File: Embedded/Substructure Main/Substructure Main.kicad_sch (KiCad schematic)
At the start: 0 parts

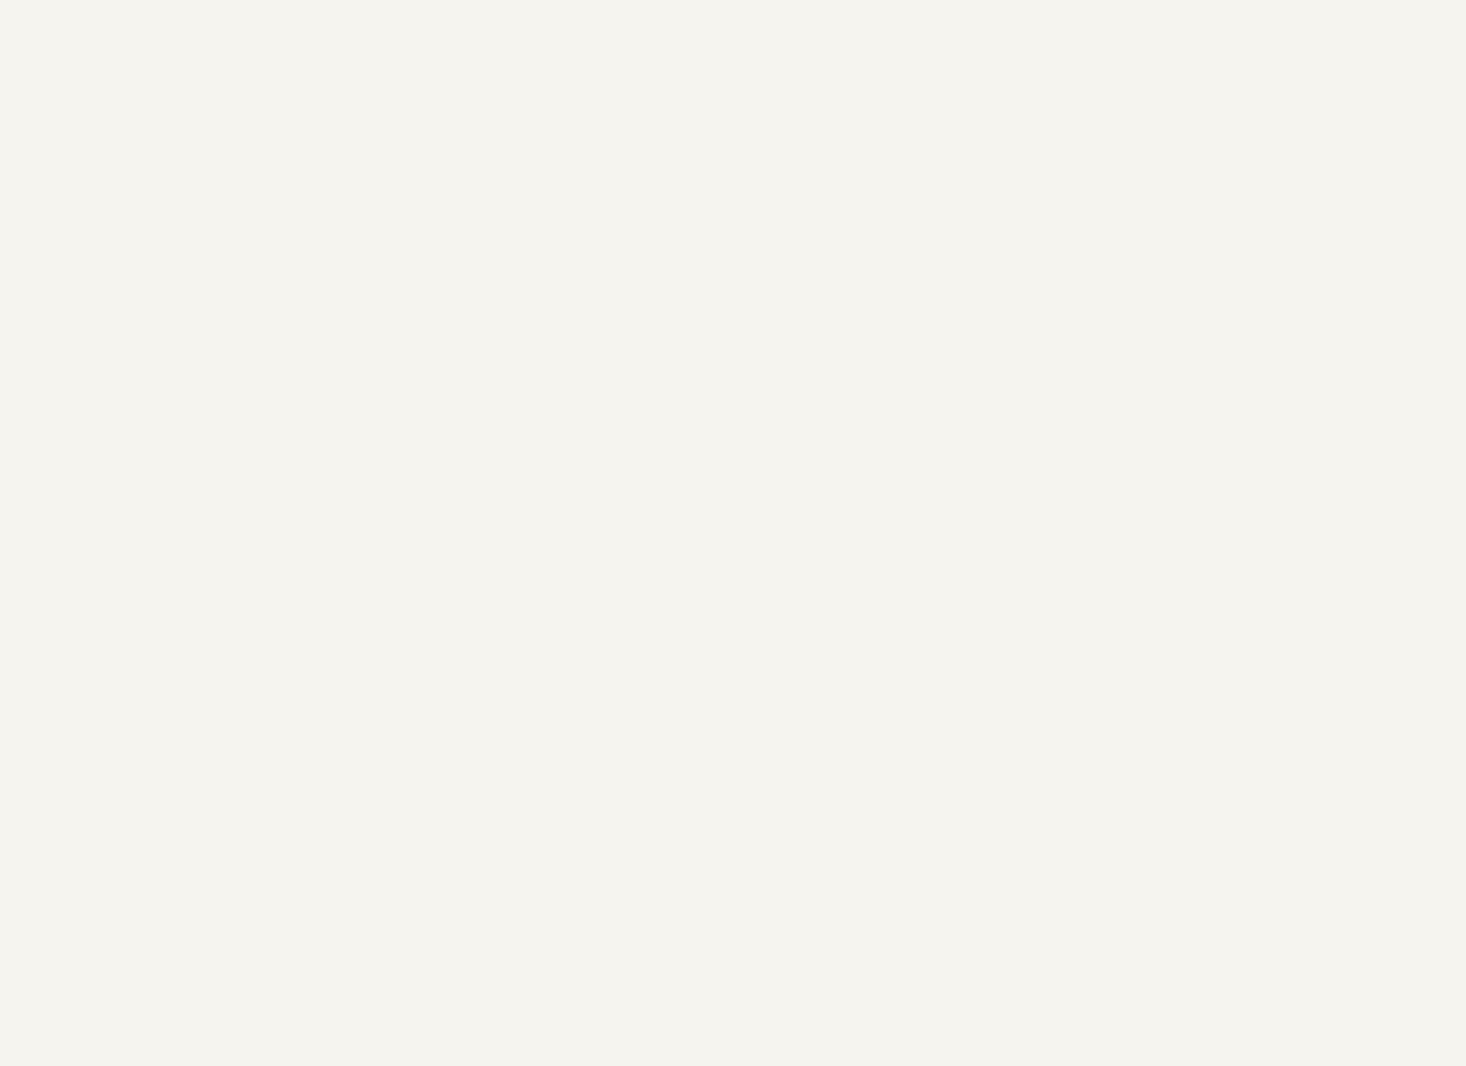
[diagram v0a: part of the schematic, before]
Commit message: Added PCB Ideation
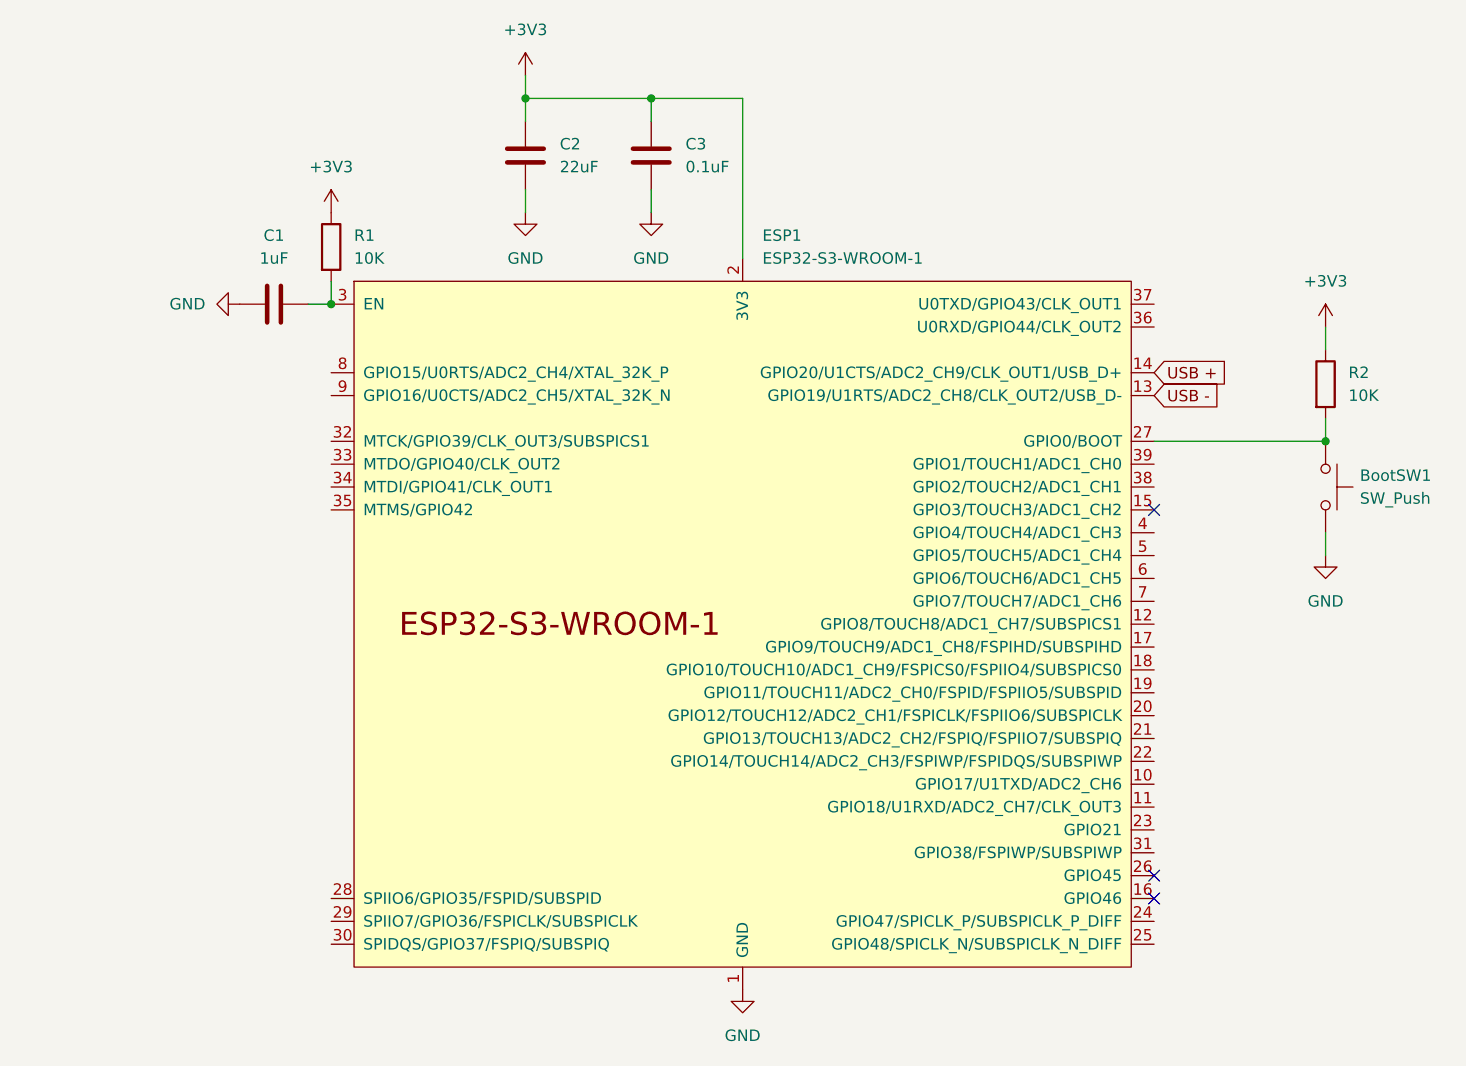
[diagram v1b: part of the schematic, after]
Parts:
- added BootSW1: SW_Push, Button-R-667843:Button-R-667843, symbol Switch:SW_Push
- added C1: 1uF, Capacitor_SMD:C_0603_1608Metric, symbol Device:C
- added C2: 22uF, Capacitor_SMD:C_0603_1608Metric_Pad1.08x0.95mm_HandSolder, symbol Device:C
- added C3: 0.1uF, Capacitor_SMD:C_0603_1608Metric_Pad1.08x0.95mm_HandSolder, symbol Device:C
- added ESP1: ESP32-S3-WROOM-1, PCM_Espressif:ESP32-S3-WROOM-1, symbol PCM_Espressif:ESP32-S3-WROOM-1
- added R1, R2: 10K, Resistor_SMD:R_0603_1608Metric, symbol Device:R
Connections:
- new net: BootSW1.1, ESP1.27 (GPIO0/BOOT), R2.2
- new net: C1.2, ESP1.3 (EN), R1.2
- new net +3V3: C2.1, C3.1, ESP1.2 (3V3), R1.1, R2.1
- new net GND: BootSW1.2, C1.1, C2.2, C3.2, ESP1.1 (GND), ESP1.40 (GND), ESP1.41 (GND)
- new net USB +: ESP1.14 (GPIO20/U1CTS/ADC2_CH9/CLK_OUT1/USB_D+)
- new net USB -: ESP1.13 (GPIO19/U1RTS/ADC2_CH8/CLK_OUT2/USB_D-)
- no-connect marks 0 -> 3
